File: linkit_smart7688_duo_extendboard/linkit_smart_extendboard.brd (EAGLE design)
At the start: 96.5 x 67.9 mm, 27 parts, among them U1 BME280

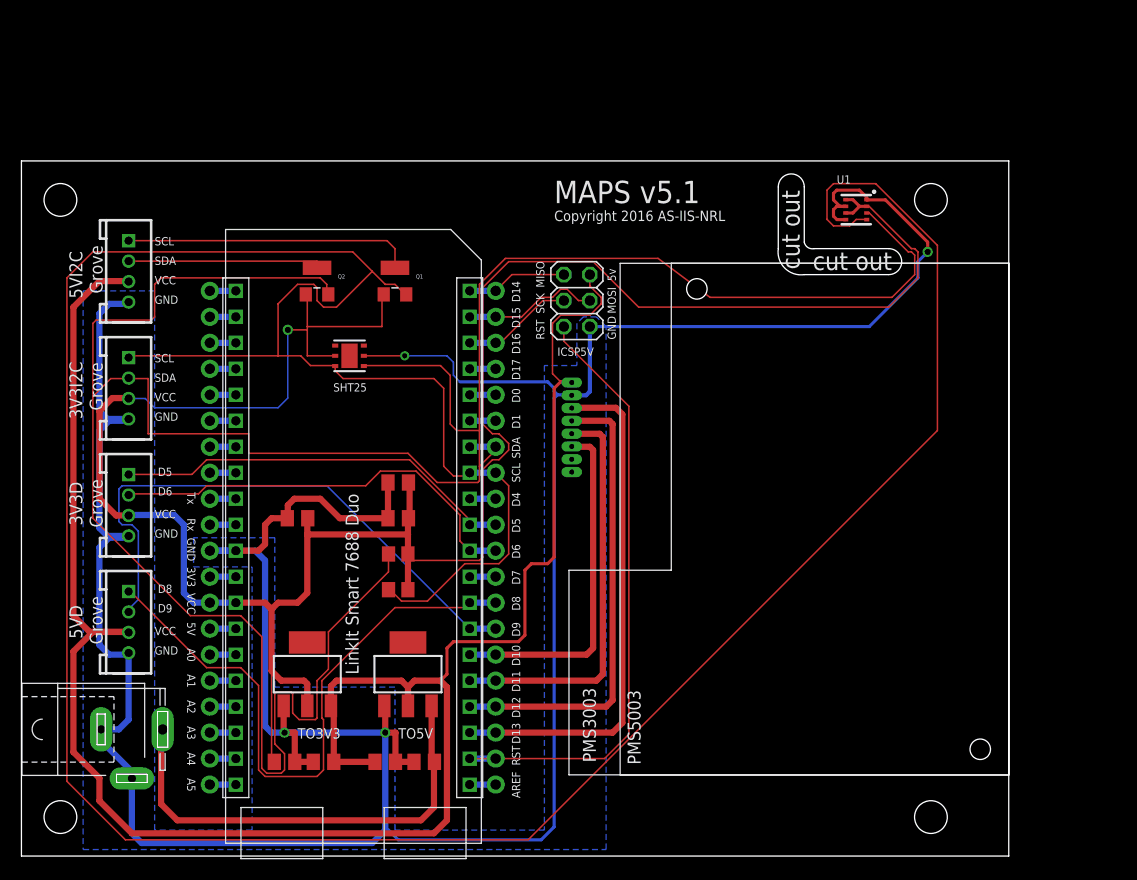
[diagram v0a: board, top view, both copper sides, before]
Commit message: revision PCB layout
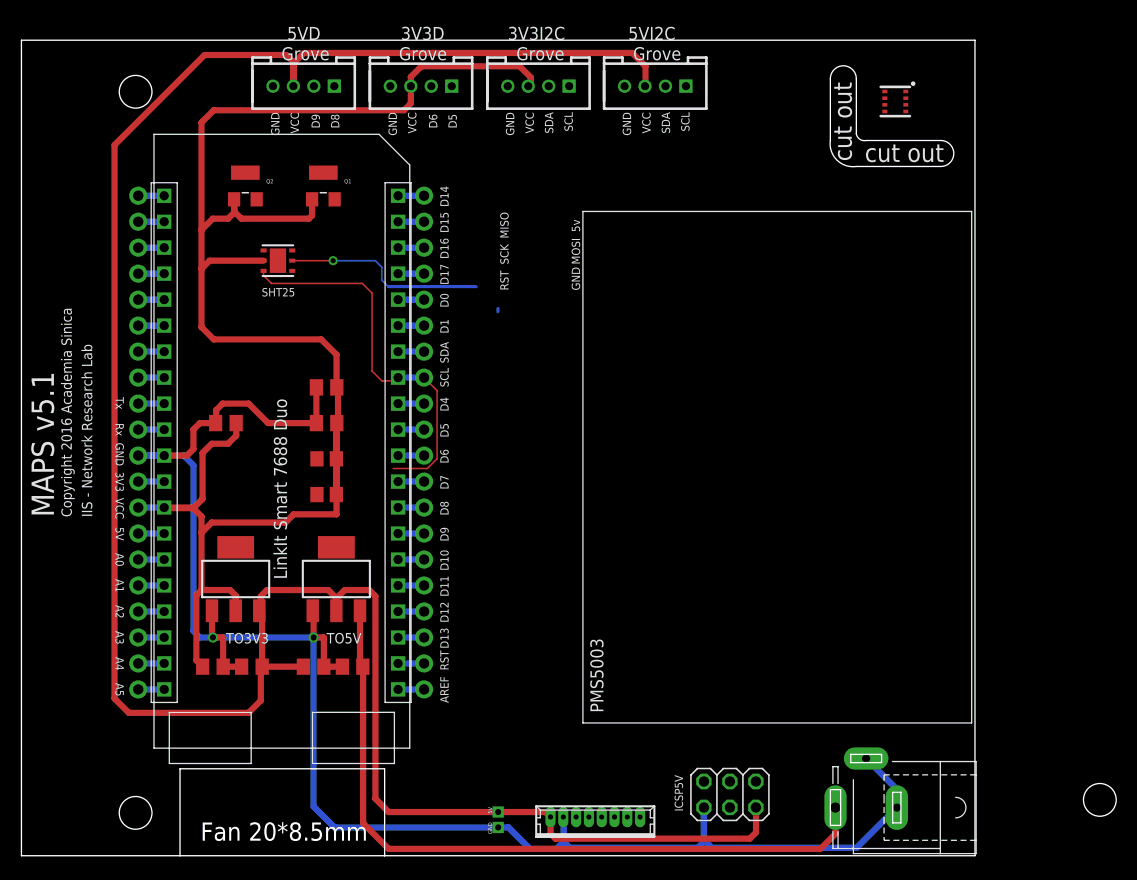
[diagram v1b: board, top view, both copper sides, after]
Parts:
- U$4: value (none) -> PIN2MM; device G3:G3 -> pin_2mm:PIN2MM
- moved POWER 72.2 mm to (82.6, 4.74), turned to 180 degrees
- moved 5VD 55.1 mm to (27.6, 75.3), turned to 180 degrees
- moved 5VI2C 54.6 mm to (62.0, 75.3), turned to 180 degrees
- moved ICSP5V 50.5 mm to (69.3, 6.02), turned to 180 degrees
- moved U$4 50.5 mm to (46.1, 4.80), turned to 270 degrees
- moved 3V3D 49.9 mm to (39.1, 75.3), turned to 180 degrees
- moved 3V3I2C 49.8 mm to (50.5, 75.3), turned to 180 degrees
- moved PMS3003 38.6 mm to (56.1, 3.37), turned to 0 degrees
- moved Q1 11.6 mm to (29.5, 65.5)
- moved Q2 11.6 mm to (21.9, 65.5)
- moved U$1 11.6 mm to (14.0, 64.5)
- moved C1 11.6 mm to (28.6, 18.5)
- moved C2 11.6 mm to (32.4, 18.5)
- moved C3 11.6 mm to (18.7, 18.5)
- moved C4 11.6 mm to (22.5, 18.5)
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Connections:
- net +5V: now also U$4.5V
- net GND: now also U$4.GND
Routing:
- net SCL: track 314.8 -> 38.5 mm
- net SDA: track 259.3 -> 2.54 mm
- net GND: track 326.6 -> 189.4 mm, vias 4 -> 3
- net +3V3: track 232.7 -> 171.6 mm, vias 1 -> 0
- net N$34: track 61.6 -> 2.54 mm
- net N$33: track 60.7 -> 2.54 mm
- net N$30: track 56.5 -> 2.54 mm
- net N$35: track 50.7 -> 2.54 mm
- net N$38: track 45.4 -> 2.54 mm
- net N$31: track 41.6 -> 2.54 mm
- net N$29: track 39.6 -> 2.54 mm
- net N$10: track 39.4 -> 2.54 mm
- net N$2: track 33.9 -> 2.54 mm
- net +5V: track 194.1 -> 224.5 mm
- net N$36: track 28.2 -> 0.00 mm
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- removed copper zone on layer 16, net GND
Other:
- board size 96.5 x 67.9 mm -> 93.2 x 79.7 mm
- board text added: "Copyright 2016 Academia Sinica"
- board text added: "Fan 20*8.5mm"
- board text added: "IIS - Network Research Lab"
- board text removed: "Copyright 2016 AS-IIS-NRL"
